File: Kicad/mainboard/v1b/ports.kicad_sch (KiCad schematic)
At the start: 14 parts, among them J3 Barrel_Jack_MountingPin, J4 SCART-F, J5 Conn_02x22_Odd_Even, J6 Conn_02x22_Odd_Even, SW2 SW_DPDT_x2

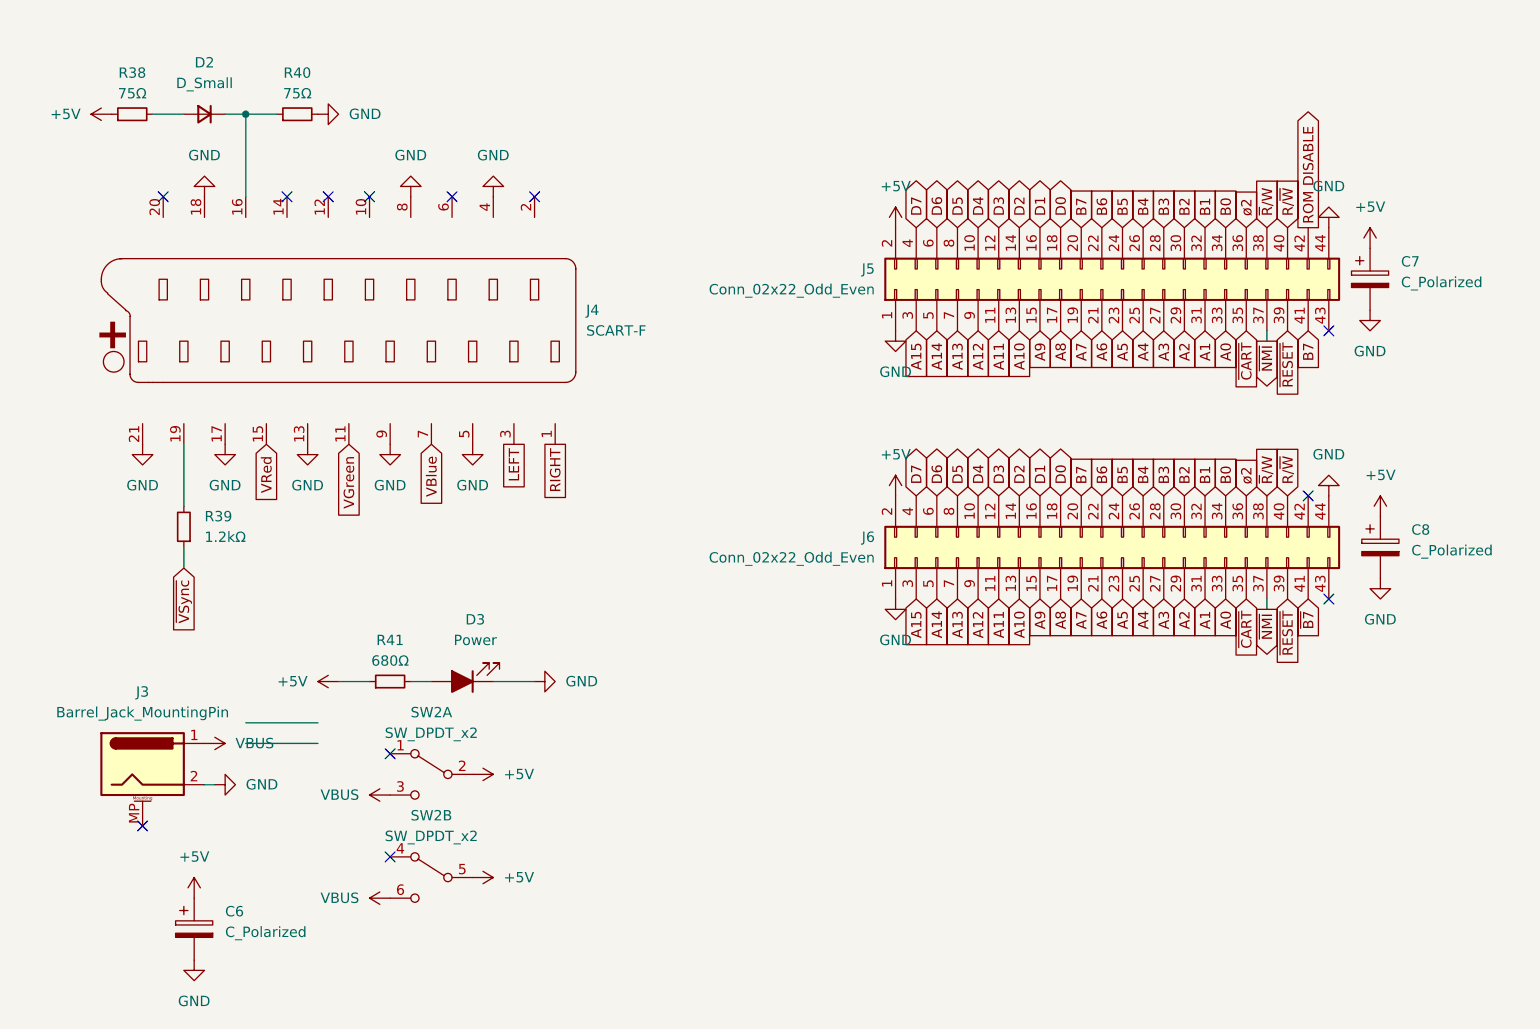
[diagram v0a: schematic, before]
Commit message: big v1b commit
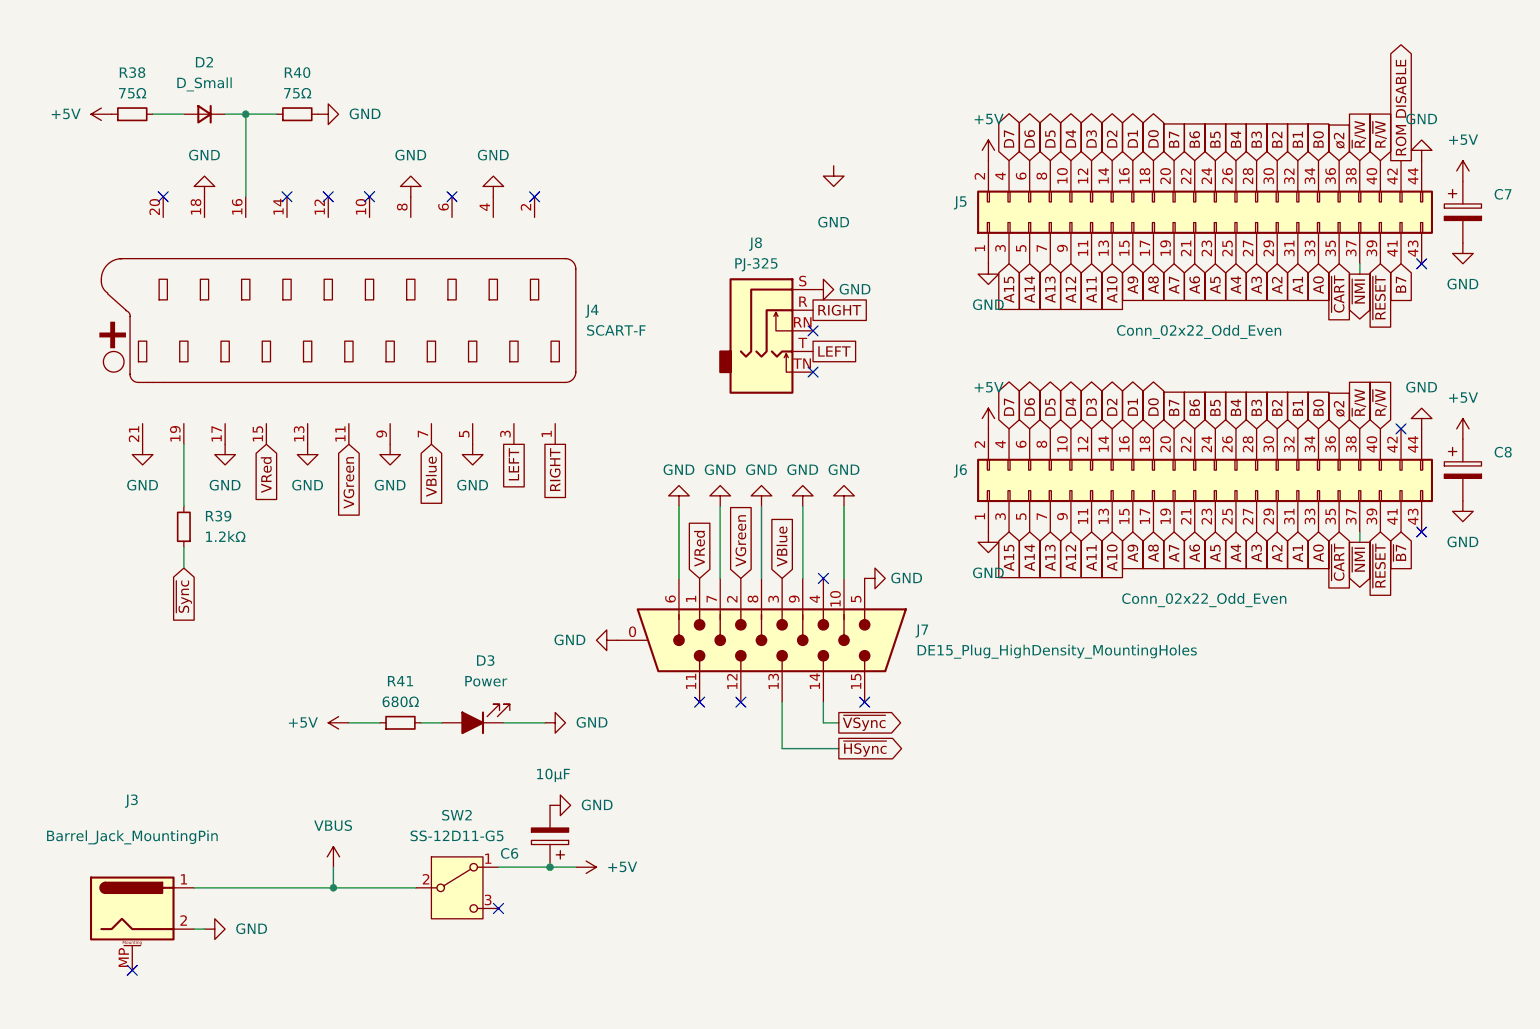
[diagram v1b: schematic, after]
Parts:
- removed SW2: SW_DPDT_x2, Button_Switch_THT:SW_CuK_JS202011AQN_DPDT_Angled, symbol Switch:SW_DPDT_x2
- added J7: DE15_Plug_HighDensity_MountingHoles, Connector_Dsub:DSUB-15-HD_Female_Horizontal_P2.29x1.98mm_EdgePinOffset8.35mm_Housed_MountingHolesOffset10.89mm, symbol Connector:DE15_Plug_HighDensity_MountingHoles
- added J8: PJ-325, Smal:Jack_3.5mm_PJ-325, symbol Connector_Audio:AudioJack3_SwitchTR
- added SW2: SS-12D11-G5, Button_Switch_THT:SW_Slide_1P2T_CK_OS102011MS2Q, symbol Switch:SW_SPDT
- C6, C7, C8: value C_Polarized -> 10µF
- D3: footprint LED_THT:LED_D5.0mm -> LED_THT:LED_Rectangular_W5.0mm_H2.0mm
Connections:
- net +5V: now also SW2.1 (A)
- net GND: now also J7.0, J7.10, J7.5, J7.6, J7.7, J7.8, J7.9, J8.S
- net LEFT: now also J8.T
- net RIGHT: now also J8.R
- net VBUS: now also SW2.2 (B)
- net VBlue: now also J7.3
- net VGreen: now also J7.2
- net VRed: now also J7.1
- net ~{VSync}: now also J7.14; no longer R39.1
- new net ~{HSync}: J7.13
- new net ~{Sync}: R39.1
- no-connect marks 12 -> 17
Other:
- moved on the sheet: C7, C8, D3, J3, J5, J6, R41
